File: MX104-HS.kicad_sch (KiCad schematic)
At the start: 57 parts, among them J1 Conn_01x03, SW1 Reset, SW2 Boot, U1 RP2040, U2 NCP1117-3.3_SOT223, U3 W25Q32JVSS, U4 Led Driver 2, U5 Led Driver 1, Y1 12MHz

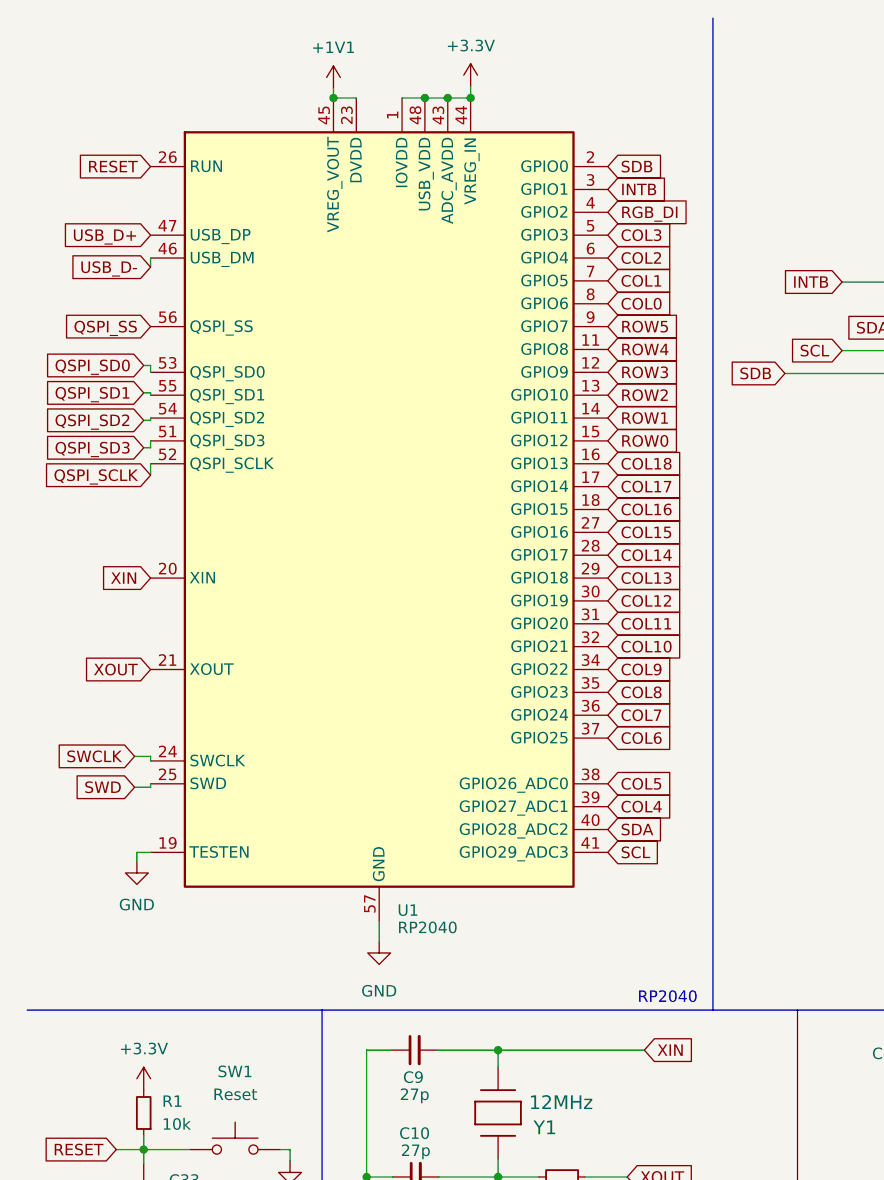
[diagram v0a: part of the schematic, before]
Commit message: Finished version 1.0
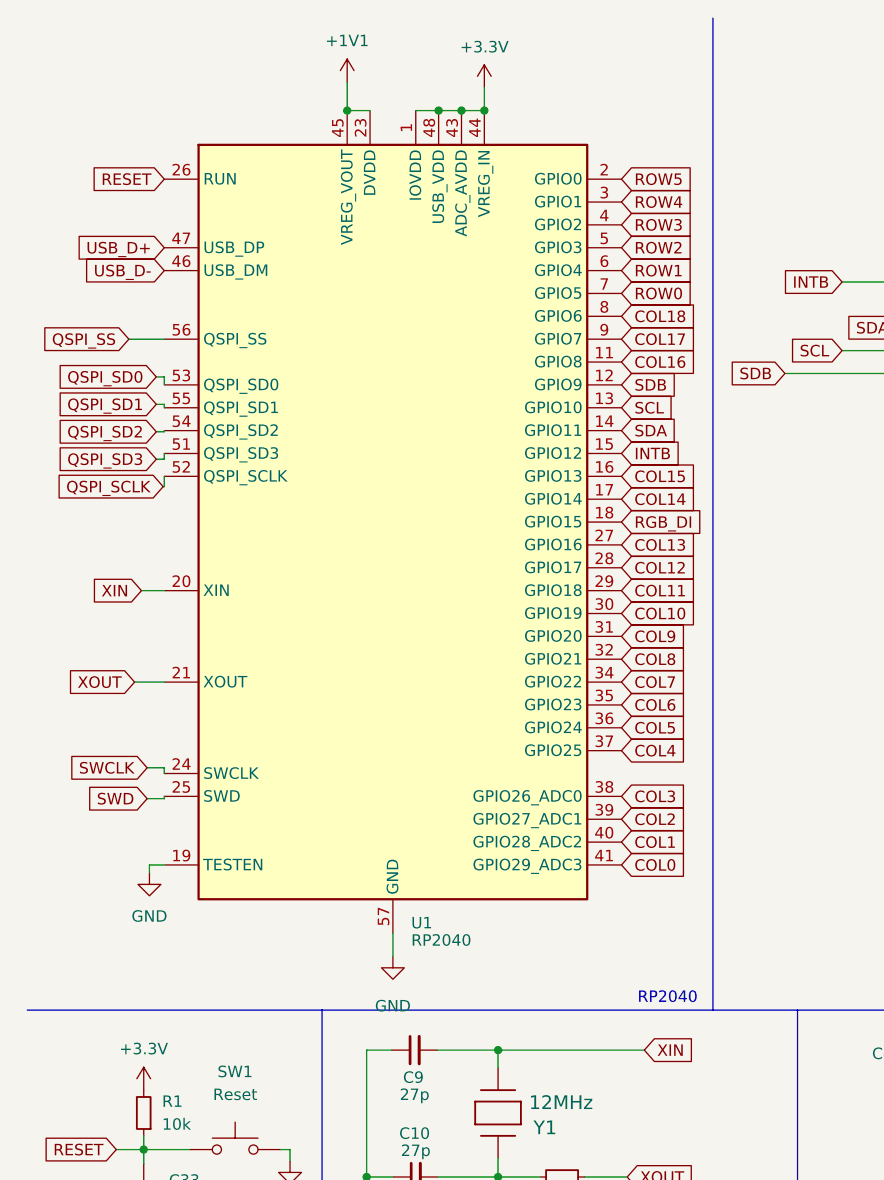
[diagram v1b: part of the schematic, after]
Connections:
- net COL0: now also U1.41 (GPIO29_ADC3); no longer U1.8 (GPIO6)
- net COL1: now also U1.40 (GPIO28_ADC2); no longer U1.7 (GPIO5)
- net COL10: now also U1.30 (GPIO19); no longer U1.32 (GPIO21)
- net COL11: now also U1.29 (GPIO18); no longer U1.31 (GPIO20)
- net COL12: now also U1.28 (GPIO17); no longer U1.30 (GPIO19)
- net COL13: now also U1.27 (GPIO16); no longer U1.29 (GPIO18)
- net COL14: now also U1.17 (GPIO14); no longer U1.28 (GPIO17)
- net COL15: now also U1.16 (GPIO13); no longer U1.27 (GPIO16)
- net COL16: now also U1.11 (GPIO8); no longer U1.18 (GPIO15)
- net COL17: now also U1.9 (GPIO7); no longer U1.17 (GPIO14)
- net COL18: now also U1.8 (GPIO6); no longer U1.16 (GPIO13)
- net COL2: now also U1.39 (GPIO27_ADC1); no longer U1.6 (GPIO4)
- net COL3: now also U1.38 (GPIO26_ADC0); no longer U1.5 (GPIO3)
- net COL4: now also U1.37 (GPIO25); no longer U1.39 (GPIO27_ADC1)
- net COL5: now also U1.36 (GPIO24); no longer U1.38 (GPIO26_ADC0)
- net COL6: now also U1.35 (GPIO23); no longer U1.37 (GPIO25)
- net COL7: now also U1.34 (GPIO22); no longer U1.36 (GPIO24)
- net COL8: now also U1.32 (GPIO21); no longer U1.35 (GPIO23)
- net COL9: now also U1.31 (GPIO20); no longer U1.34 (GPIO22)
- net INTB: now also U1.15 (GPIO12); no longer U1.3 (GPIO1)
- net RGB_DI: now also U1.18 (GPIO15); no longer U1.4 (GPIO2)
- net ROW0: now also U1.7 (GPIO5); no longer U1.15 (GPIO12)
- net ROW1: now also U1.6 (GPIO4); no longer U1.14 (GPIO11)
- net ROW2: now also U1.5 (GPIO3); no longer U1.13 (GPIO10)
- net ROW3: now also U1.4 (GPIO2); no longer U1.12 (GPIO9)
- net ROW4: now also U1.3 (GPIO1); no longer U1.11 (GPIO8)
- net ROW5: now also U1.2 (GPIO0); no longer U1.9 (GPIO7)
- net SCL: now also U1.13 (GPIO10); no longer U1.41 (GPIO29_ADC3)
- net SDA: now also U1.14 (GPIO11); no longer U1.40 (GPIO28_ADC2)
- net SDB: now also U1.12 (GPIO9); no longer U1.2 (GPIO0)
